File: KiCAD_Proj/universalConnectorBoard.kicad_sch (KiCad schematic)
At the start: 29 parts, among them IC1 RPI_Pico_EvaluationBoard, IC2 SN74LV4052ADR, IC4 TCA9534DWR, J2 Display1, J3 Display2, J4 RPI4, J5 Ledstrip2, J6 MUX3_UART, J7 MUX4_UART, J8 Ledstrip1, U3 TMC2209_MotorDriver, U4 TMC2209_MotorDriver

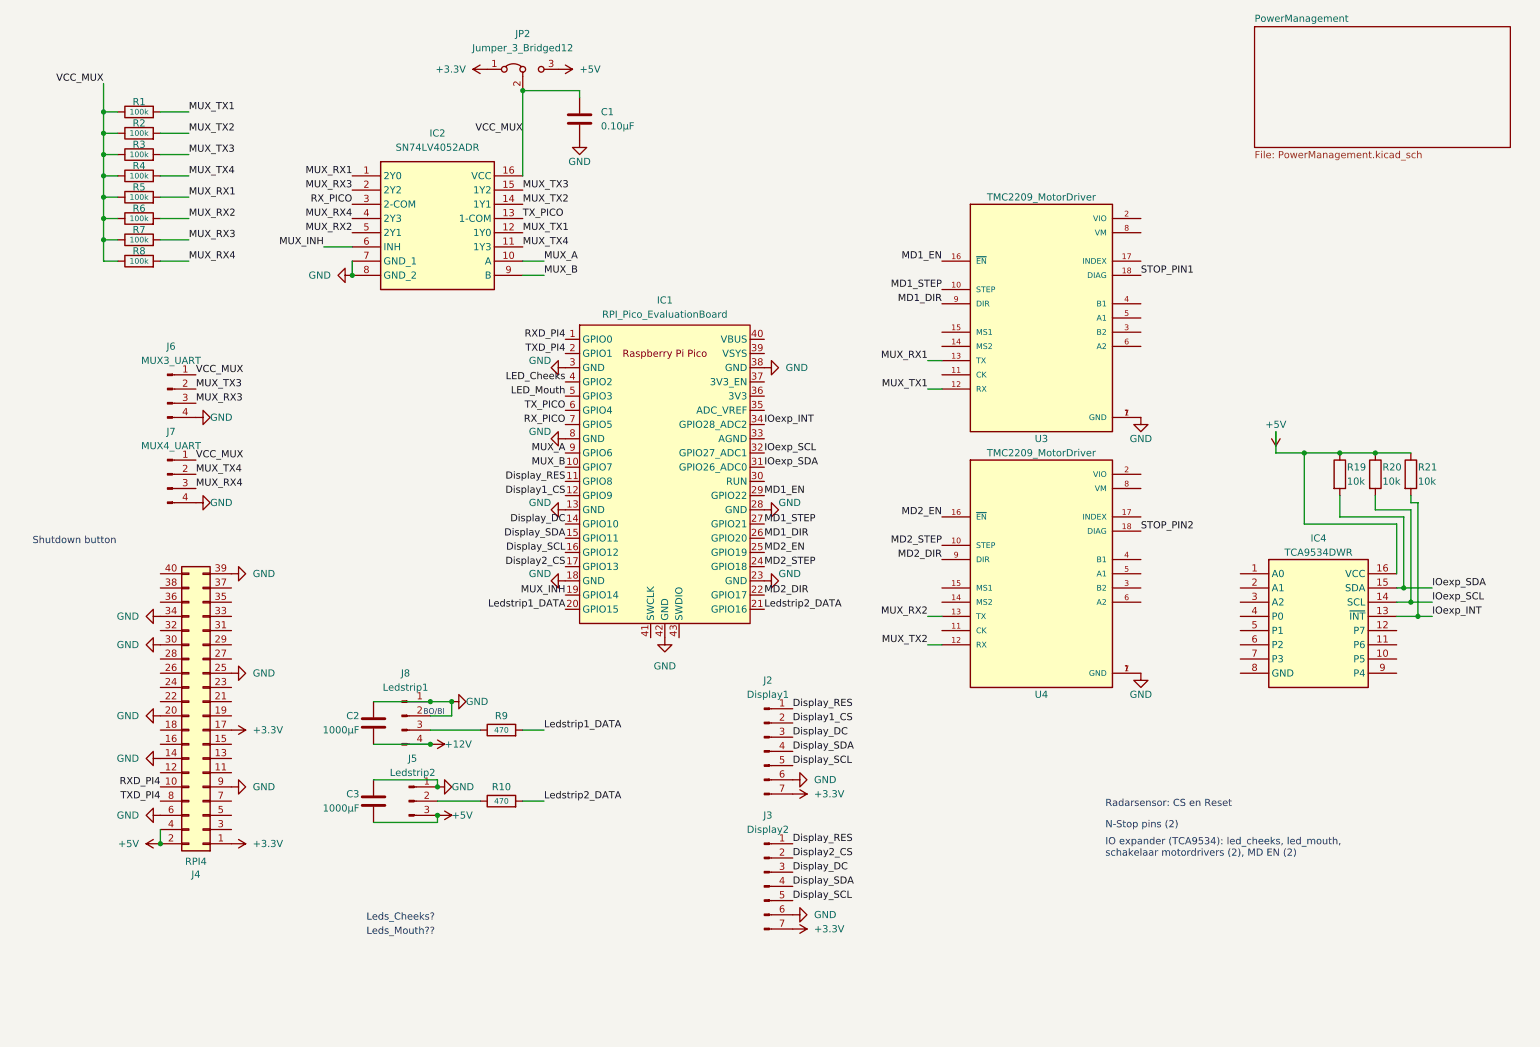
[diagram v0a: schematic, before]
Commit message: Schematic nearly done, ordened
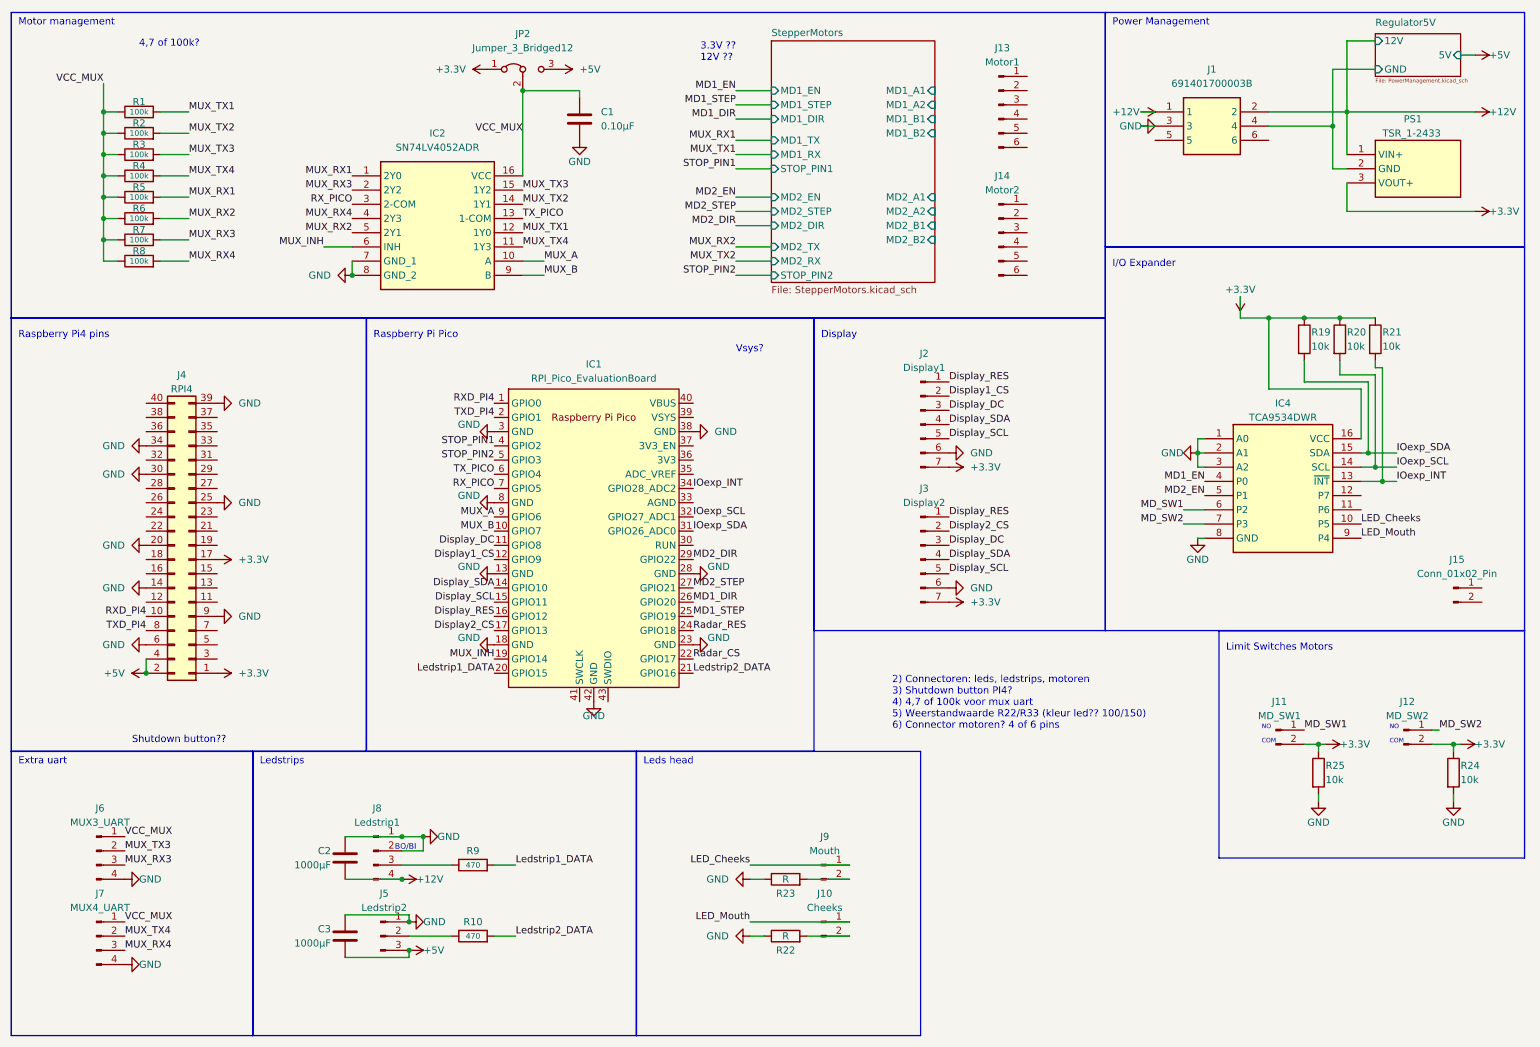
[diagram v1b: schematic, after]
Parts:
- removed U3, U4: TMC2209_MotorDriver, TMC2209_SILENTSTEPSTICK:MODULE_TMC2209_SILENTSTEPSTICK, symbol projectLib:TMC2209_MotorDriver
- added J1: 691401700003B, SamacSys_Parts:691401700003B, symbol Healthbot-Symbols:Terminal_Block3
- added J10: Cheeks, Connector_JST:JST_XH_S2B-XH-A_1x02_P2.50mm_Horizontal, symbol Connector:Conn_01x02_Pin
- added J11: MD_SW1, Connector_JST:JST_XH_S2B-XH-A_1x02_P2.50mm_Horizontal, symbol Connector:Conn_01x02_Pin
- added J12: MD_SW2, Connector_JST:JST_XH_S2B-XH-A_1x02_P2.50mm_Horizontal, symbol Connector:Conn_01x02_Pin
- added J13: Motor1, Connector_JST:JST_XH_S6B-XH-A_1x06_P2.50mm_Horizontal, symbol Connector:Conn_01x06_Pin
- added J14: Motor2, Connector_JST:JST_XH_S6B-XH-A_1x06_P2.50mm_Horizontal, symbol Connector:Conn_01x06_Pin
- added J15: Conn_01x02_Pin, symbol Connector:Conn_01x02_Pin
- added J9: Mouth, Connector_JST:JST_XH_S2B-XH-A_1x02_P2.50mm_Horizontal, symbol Connector:Conn_01x02_Pin
- added PS1: TSR_1-2433, SamacSys_Parts:TSR-1-2433, symbol Healthbot-Symbols:DC-DC_3.3V
- added R22, R23: R, Resistor_SMD:R_0603_1608Metric_Pad0.98x0.95mm_HandSolder, symbol Device:R
- added R24, R25: 10k, Resistor_SMD:R_0603_1608Metric_Pad0.98x0.95mm_HandSolder, symbol Device:R
- IC4: footprint SOIC127P1030X265-16N -> SamacSys_Parts:SOIC127P1030X265-16N
- R19, R20, R21: footprint (none) -> Resistor_SMD:R_0603_1608Metric_Pad0.98x0.95mm_HandSolder
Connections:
- net +12V: now also J1.1, J1.2, PS1.1 (VIN+)
- net +3.3V: now also IC4.16 (VCC), R19.1, R20.1, R21.1, J11.2 (Pin_2), J12.2 (Pin_2), PS1.3 (VOUT+), R24.1, R25.1
- net +5V: no longer IC4.16 (VCC), R19.1, R20.1, R21.1
- net Display_DC: now also IC1.11 (GPIO8); no longer IC1.14 (GPIO10)
- net Display_RES: now also IC1.16 (GPIO12); no longer IC1.11 (GPIO8)
- net Display_SCL: now also IC1.15 (GPIO11); no longer IC1.16 (GPIO12)
- net Display_SDA: now also IC1.14 (GPIO10); no longer IC1.15 (GPIO11)
- net GND: now also IC4.1 (A0), IC4.2 (A1), IC4.3 (A2), IC4.8 (GND), J1.3, R22.1, R23.1, R24.2, R25.2
- net LED_Cheeks: now also IC4.10 (P5), J9.1 (Pin_1); no longer IC1.4 (GPIO2)
- net LED_Mouth: now also IC4.9 (P4), J10.1 (Pin_1); no longer IC1.5 (GPIO3)
- net MD1_EN: now also IC4.4 (P0); no longer IC1.29 (GPIO22)
- net MD1_STEP: now also IC1.25 (GPIO19); no longer IC1.27 (GPIO21)
- net MD2_DIR: now also IC1.29 (GPIO22); no longer IC1.22 (GPIO17)
- net MD2_EN: now also IC4.5 (P1); no longer IC1.25 (GPIO19)
- net MD2_STEP: now also IC1.27 (GPIO21); no longer IC1.24 (GPIO18)
- net STOP_PIN1: now also IC1.4 (GPIO2)
- net STOP_PIN2: now also IC1.5 (GPIO3)
- net MD_SW1: now reaches IC4.6 (P2)
- net MD_SW1: now also J11.1 (Pin_1)
- net MD_SW2: now reaches IC4.7 (P3)
- net MD_SW2: now also J12.1 (Pin_1)
- new net: J9.2 (Pin_2), R23.2
- new net: J10.2 (Pin_2), R22.2
- new net Radar_CS: IC1.22 (GPIO17)
- new net Radar_RES: IC1.24 (GPIO18)
- new net Regulator5V/GND: J1.4, PS1.2 (GND)
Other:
- sheet PowerManagement renamed Regulator5V
- added sheet StepperMotors (StepperMotors.kicad_sch)
- sheet Regulator5V ports: added 12V, 5V, GND; removed none
- note added: "2) Connectoren: leds, ledstrips, motoren 3) Shutdown button PI4? 4) 4,7 of 100k voor mux uart 5) Weerstandwaarde R22/R33 (kleur led?? 100/150) 6) Connector motoren? 4 of 6 pins"
- note added: "3.3V ?? 12V ??"
- note added: "4,7 of 100k?"
- note added: "COM"
- note added: "Display"
- note added: "Extra uart"
- note added: "I/O Expander"
- note added: "Leds head"
- note added: "Ledstrips"
- note added: "Limit Switches Motors"
- note added: "Motor management"
- note added: "NO"
- note added: "Power Management"
- note added: "Raspberry Pi Pico"
- note added: "Raspberry Pi4 pins"
- note added: "Shutdown button??"
- note added: "Vsys?"
- note removed: "IO expander (TCA9534): led_cheeks, led_mouth, schakelaar motordrivers (2), MD EN (2)"
- note removed: "Leds_Cheeks?"
- note removed: "Leds_Mouth??"
- note removed: "N-Stop pins (2)"
- note removed: "Radarsensor: CS en Reset"
- note removed: "Shutdown button"
- company: (none) -> HAN Univeristy of Applied Sciences
- title: (none) -> Project_Healthbot_HAT
- moved on the sheet: C2, C3, IC1, IC4, J2, J3, J4, J5, J6, J7, J8, R10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
